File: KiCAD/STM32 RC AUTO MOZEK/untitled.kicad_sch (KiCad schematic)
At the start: 25 parts, among them J3 Conn_01x05_Socket, J4 Conn_01x03_Socket, J5 Conn_01x03_Socket, J6 Conn_01x02_Socket, J7 Conn_01x02_Socket, Q1 SI2312, Q2 SI2312, Q3 SI2312, Q4 SI2312, SW1 SW_Push, U12 NRF24L01_Breakout, U13 STM32F411RCTx, Y3 25MHz, Y4 32.786KHz

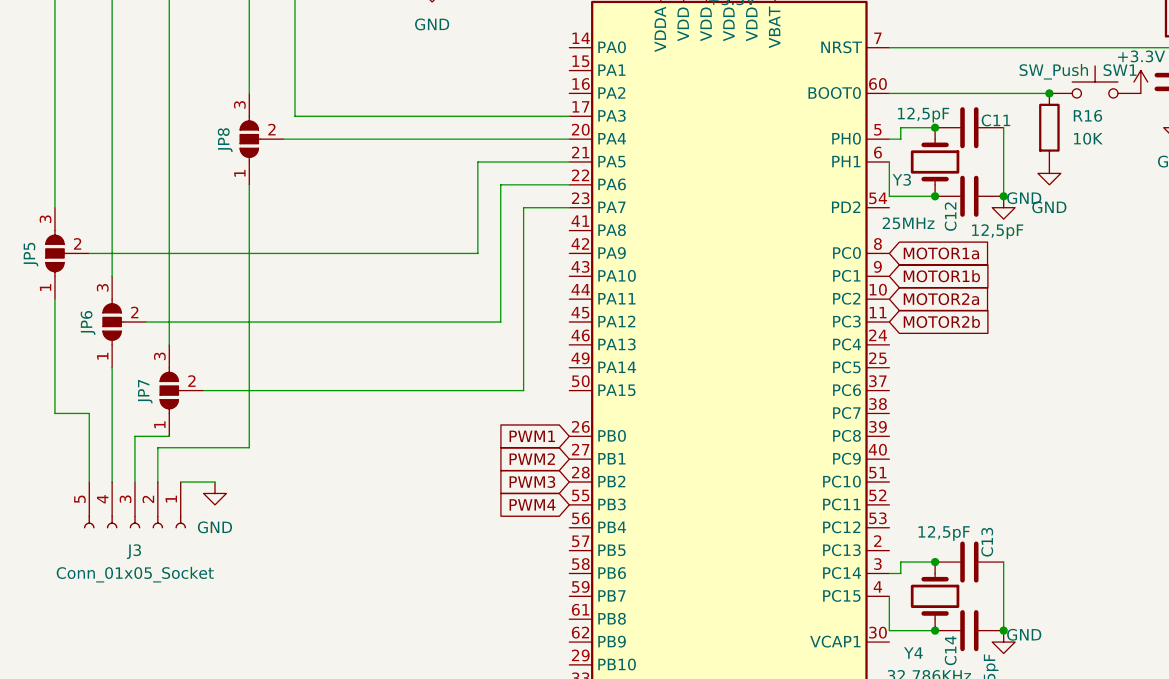
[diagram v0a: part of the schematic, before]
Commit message: .
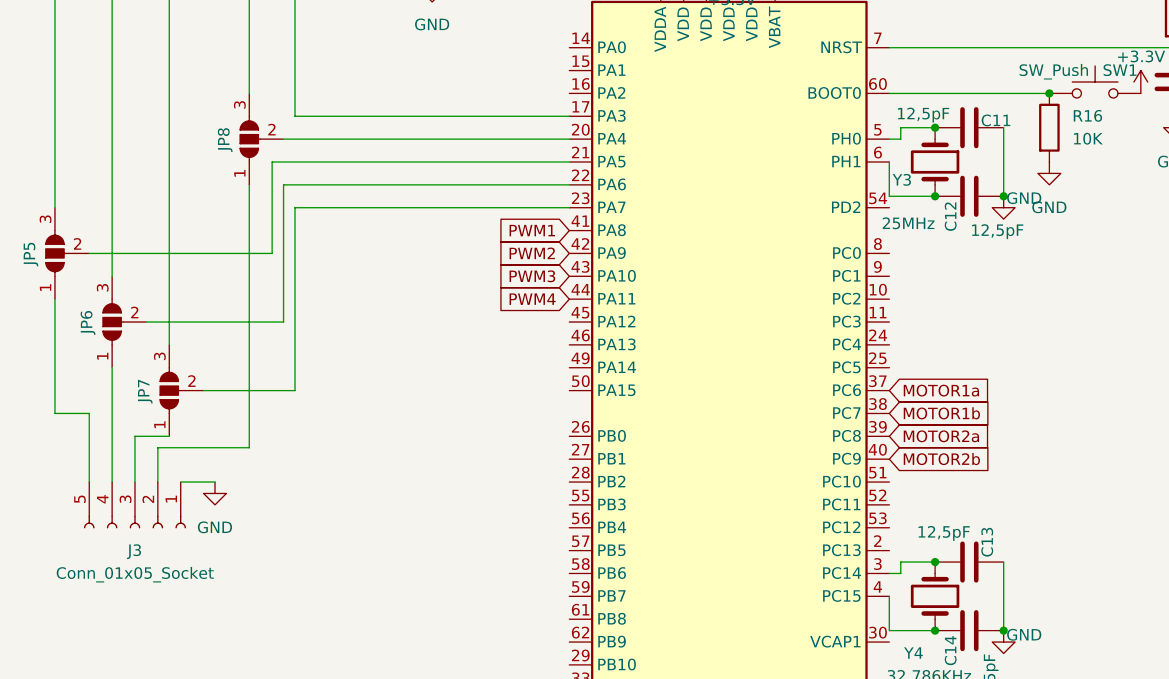
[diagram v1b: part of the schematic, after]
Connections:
- net MOTOR1a: now also U13.37 (PC6); no longer U13.8 (PC0)
- net MOTOR1b: now also U13.38 (PC7); no longer U13.9 (PC1)
- net MOTOR2a: now also U13.39 (PC8); no longer U13.10 (PC2)
- net MOTOR2b: now also U13.40 (PC9); no longer U13.11 (PC3)
- net PWM1: now also U13.41 (PA8); no longer U13.26 (PB0)
- net PWM2: now also U13.42 (PA9); no longer U13.27 (PB1)
- net PWM3: now also U13.43 (PA10); no longer U13.28 (PB2)
- net PWM4: now also U13.44 (PA11); no longer U13.55 (PB3)
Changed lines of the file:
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@@
 	(wire
 		(pts
-			(xy 78.74 68.58) (xy 86.36 68.58)
+			(xy 54.61 68.58) (xy 86.36 68.58)
 		)
 		(stroke
@@
 	(wire
 		(pts
-			(xy 39.37 83.82) (xy 78.74 83.82)
+			(xy 39.37 83.82) (xy 54.61 83.82)
 		)
 		(stroke
@@
 	(wire
 		(pts
-			(xy 76.2 66.04) (xy 86.36 66.04)
+			(xy 53.34 66.04) (xy 86.36 66.04)
 		)
 		(stroke
@@
 	(wire
 		(pts
-			(xy 45.72 91.44) (xy 81.28 91.44)
-		)
-		(stroke
-			(width 0)
-			(type default)
-		)
-	)
-	(wire
-		(pts
-			(xy 78.74 83.82) (xy 78.74 68.58)
+			(xy 45.72 91.44) (xy 55.88 91.44)
+		)
+		(stroke
+			(width 0)
+			(type default)
+		)
+	)
+	(wire
+		(pts
+			(xy 54.61 83.82) (xy 54.61 68.58)
 		)
 		(stroke
@@
 	(wire
 		(pts
-			(xy 33.02 76.2) (xy 76.2 76.2)
+			(xy 33.02 76.2) (xy 53.34 76.2)
 		)
 		(stroke
@@
 	(wire
 		(pts
-			(xy 76.2 76.2) (xy 76.2 66.04)
+			(xy 53.34 76.2) (xy 53.34 66.04)
 		)
 		(stroke
@@
 	(wire
 		(pts
-			(xy 81.28 71.12) (xy 86.36 71.12)
+			(xy 55.88 71.12) (xy 86.36 71.12)
 		)
 		(stroke
@@
 	(wire
 		(pts
-			(xy 81.28 91.44) (xy 81.28 71.12)
+			(xy 55.88 91.44) (xy 55.88 71.12)
 		)
 		(stroke
@@
 	(global_label "PWM3"
 		(shape input)
-		(at 86.36 101.6 180)
+		(at 86.36 78.74 180)
 		(fields_autoplaced yes)
 		(effects
@@
 		)
 		(property "Intersheetrefs" "${INTERSHEET_REFS}"
-			(at 77.9925 101.6 0)
+			(at 77.9925 78.74 0)
 			(effects
 				(font
@@
 	(global_label "MOTOR2b"
 		(shape input)
-		(at 121.92 83.82 0)
+		(at 121.92 99.06 0)
 		(fields_autoplaced yes)
 		(effects
@@
 		)
 		(property "Intersheetrefs" "${INTERSHEET_REFS}"
-			(at 133.6137 83.82 0)
+			(at 133.6137 99.06 0)
 			(effects
 				(font
@@
 	(global_label "MOTOR1b"
 		(shape input)
-		(at 121.92 78.74 0)
+		(at 121.92 93.98 0)
 		(fields_autoplaced yes)
 		(effects
@@
 		)
 		(property "Intersheetrefs" "${INTERSHEET_REFS}"
-			(at 133.6137 78.74 0)
+			(at 133.6137 93.98 0)
 			(effects
 				(font
@@
 	(global_label "PWM2"
 		(shape input)
-		(at 86.36 99.06 180)
+		(at 86.36 76.2 180)
 		(fields_autoplaced yes)
 		(effects
@@
 		)
 		(property "Intersheetrefs" "${INTERSHEET_REFS}"
-			(at 77.9925 99.06 0)
+			(at 77.9925 76.2 0)
 			(effects
 				(font
@@
 	(global_label "MOTOR1a"
 		(shape input)
-		(at 121.92 76.2 0)
+		(at 121.92 91.44 0)
 		(fields_autoplaced yes)
 		(effects
@@
 		)
 		(property "Intersheetrefs" "${INTERSHEET_REFS}"
-			(at 133.6137 76.2 0)
+			(at 133.6137 91.44 0)
 			(effects
 				(font
@@
 	(global_label "MOTOR2a"
 		(shape input)
-		(at 121.92 81.28 0)
+		(at 121.92 96.52 0)
 		(fields_autoplaced yes)
 		(effects
@@
 		)
 		(property "Intersheetrefs" "${INTERSHEET_REFS}"
-			(at 133.6137 81.28 0)
+			(at 133.6137 96.52 0)
 			(effects
 				(font
@@
 	(global_label "PWM4"
 		(shape input)
-		(at 86.36 104.14 180)
+		(at 86.36 81.28 180)
 		(fields_autoplaced yes)
 		(effects
@@
 		)
 		(property "Intersheetrefs" "${INTERSHEET_REFS}"
-			(at 77.9925 104.14 0)
+			(at 77.9925 81.28 0)
 			(effects
 				(font
@@
 	(global_label "PWM1"
 		(shape input)
-		(at 86.36 96.52 180)
+		(at 86.36 73.66 180)
 		(fields_autoplaced yes)
 		(effects
@@
 		)
 		(property "Intersheetrefs" "${INTERSHEET_REFS}"
-			(at 77.9925 96.52 0)
-			(effects
-				(font
+			(at 77.9925 73.66 0)
+			(effects
+				(font
